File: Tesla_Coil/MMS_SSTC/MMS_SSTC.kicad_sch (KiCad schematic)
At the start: 57 parts, among them J1 Screw_Terminal_01x02, J2 Screw_Terminal_01x02, J3 Screw_Terminal_01x02, J4 Screw_Terminal_01x02, Q1 IRFP460APBF, U1 LM7812_TO220, U2 LM7805_TO220, U3 CD74HC14E, U4 UCC27524P, U5 NE555P

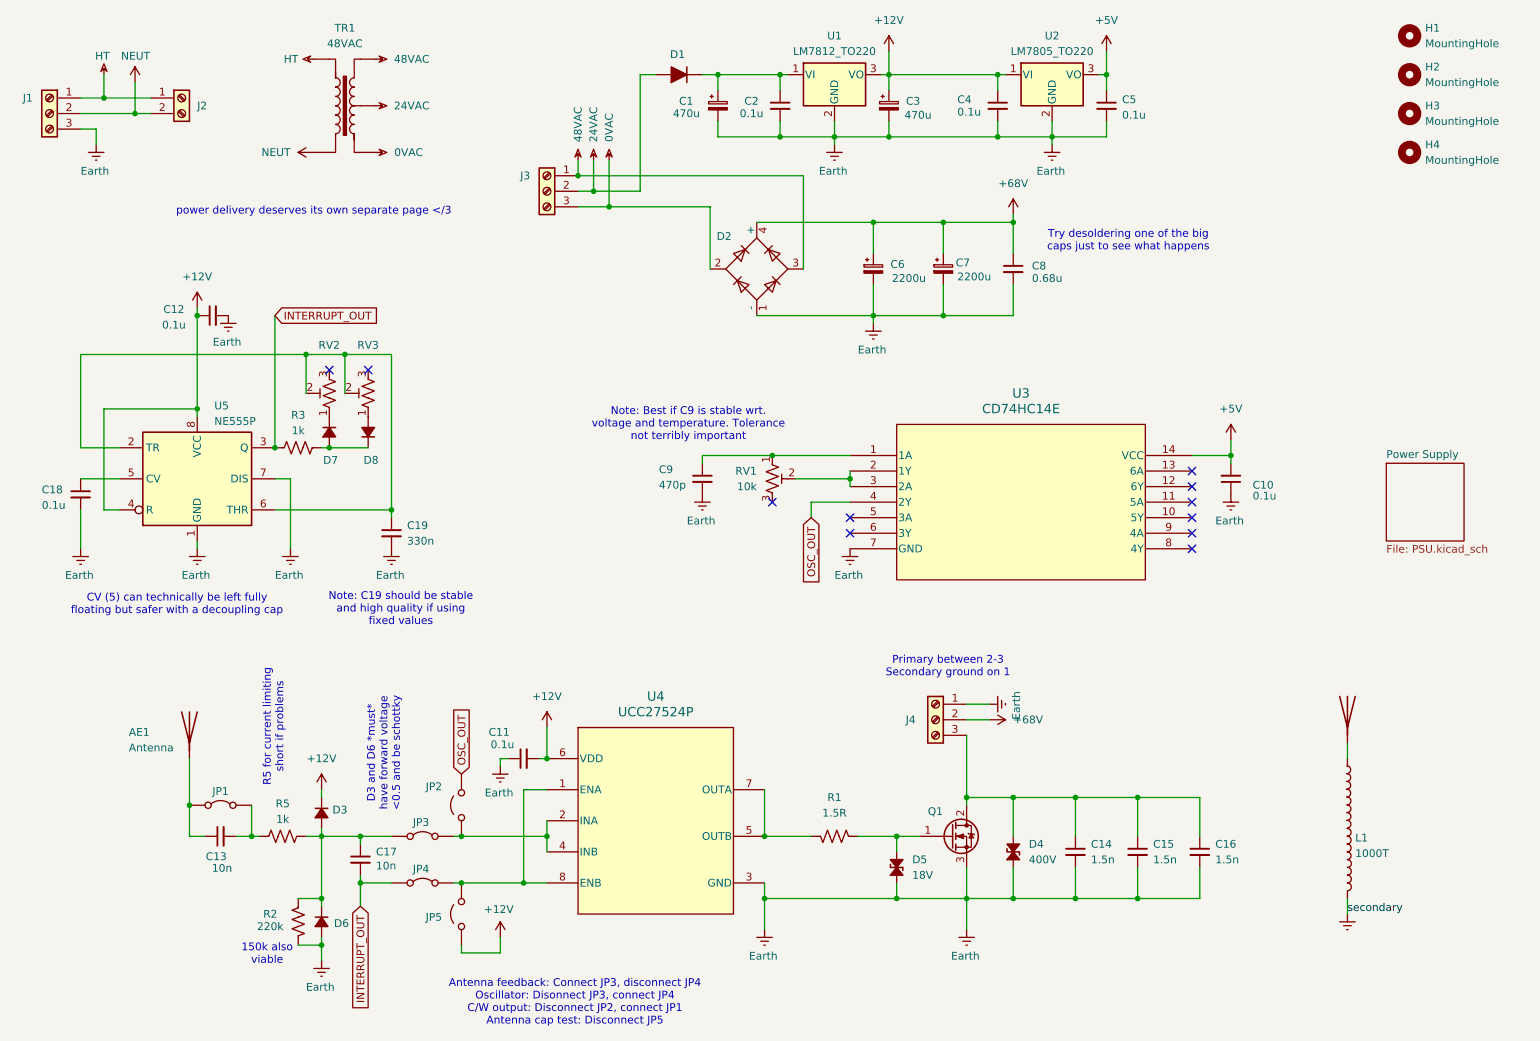
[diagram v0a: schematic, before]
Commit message: Begin work on final tesla coil design
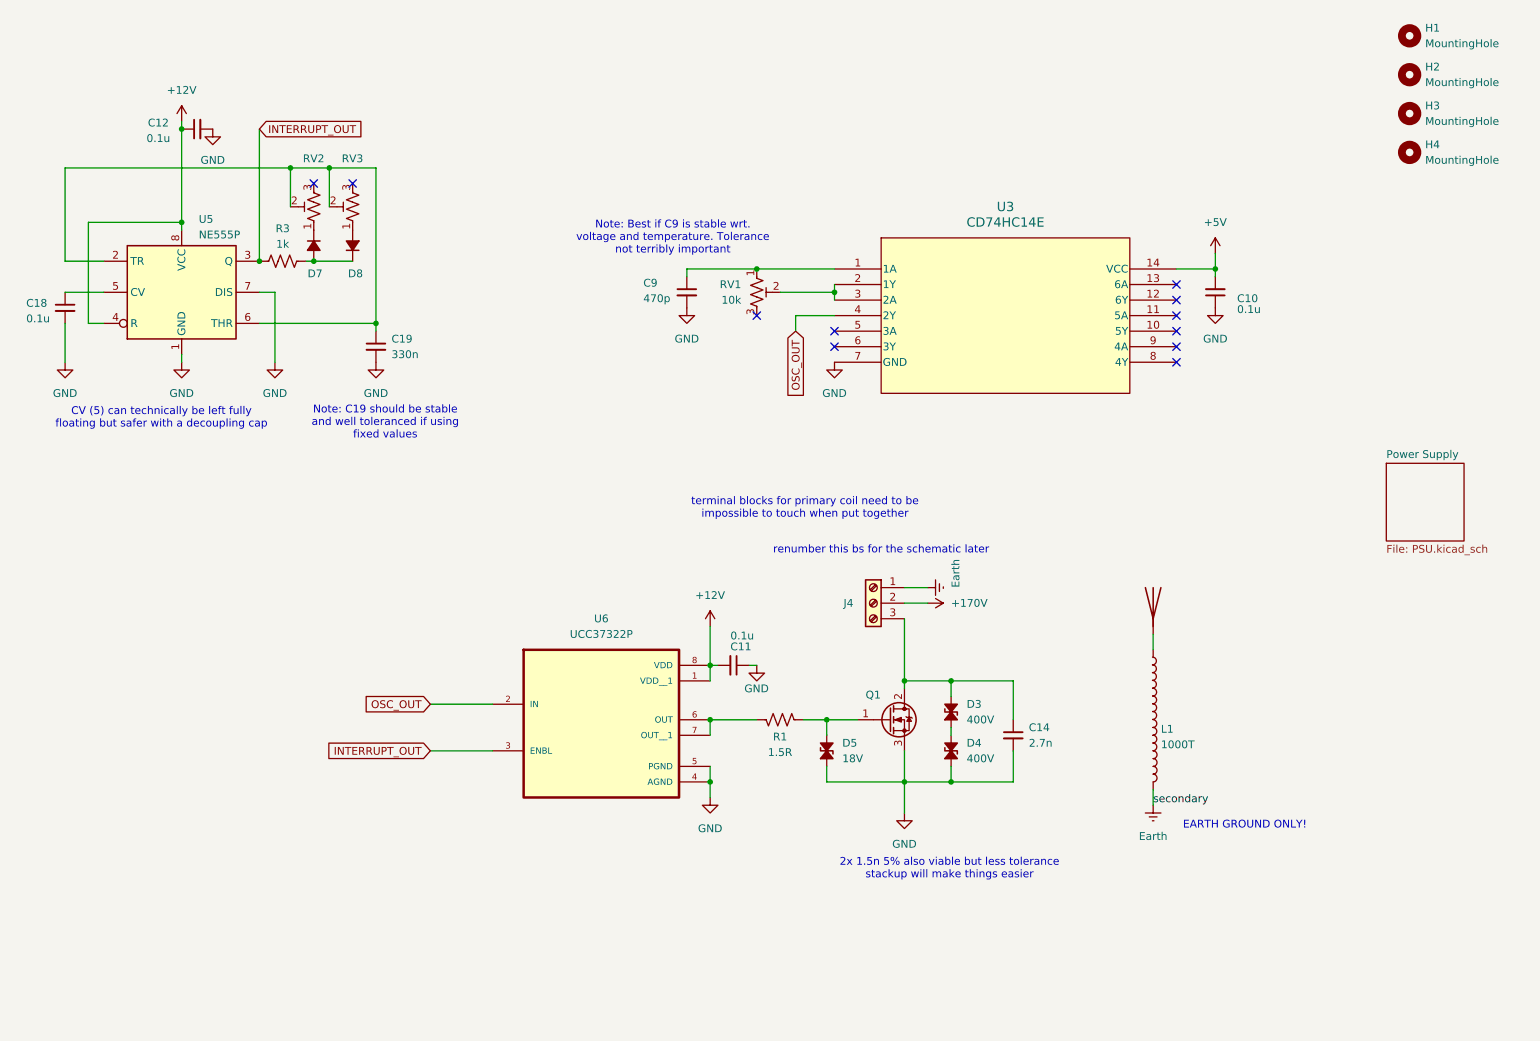
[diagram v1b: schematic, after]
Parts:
- removed AE1: Antenna, TestPoint:TestPoint_Keystone_5000-5004_Miniature, symbol Device:Antenna
- removed C1, C3: 470u, Capacitor_THT:CP_Radial_D12.5mm_P5.00mm, symbol Device:C_Polarized_Small
- removed C13, C17: 10n, Capacitor_THT:C_Disc_D5.0mm_W2.5mm_P2.50mm, symbol Device:C_Small
- removed C15, C16: 1.5n, Capacitor_THT:C_Rect_L13.0mm_W4.0mm_P10.00mm_FKS3_FKP3_MKS4, symbol Device:C_Small
- removed C2, C4, C5: 0.1u, Capacitor_THT:C_Disc_D3.0mm_W2.0mm_P2.50mm, symbol Device:C_Small
- removed C6, C7: 2200u, Capacitor_THT:CP_Radial_D25.0mm_P10.00mm_SnapIn, symbol Device:C_Polarized_Small
- removed C8: 0.68u, Capacitor_THT:C_Rect_L7.2mm_W5.5mm_P5.00mm_FKS2_FKP2_MKS2_MKP2, symbol Device:C_Small
- removed D1: D_Filled, Diode_THT:D_DO-41_SOD81_P7.62mm_Horizontal, symbol Device:D_Filled
- removed D2: B125C2300-1500A, Diode_THT:Diode_Bridge_Vishay_GBU, symbol Diode_Bridge:B125C2300-1500A
- removed D3, D6: ~, Diode_THT:D_DO-41_SOD81_P7.62mm_Horizontal, symbol Device:D_Small_Filled
- removed J1, J3: Screw_Terminal_01x02, locals:691137710003, symbol Connector:Screw_Terminal_01x03
- removed J2: Screw_Terminal_01x02, locals:691137710002, symbol Connector:Screw_Terminal_01x02
- removed JP1, JP3, JP4: Jumper_2_Bridged, TestPoint:TestPoint_Bridge_Pitch2.54mm_Drill0.7mm, symbol Jumper:Jumper_2_Bridged
- removed JP2, JP5: Jumper_2_Open, TestPoint:TestPoint_Bridge_Pitch2.54mm_Drill0.7mm, symbol Jumper:Jumper_2_Open
- removed R2: 220k, Resistor_THT:R_Axial_DIN0204_L3.6mm_D1.6mm_P5.08mm_Horizontal, symbol Device:R_US
- removed R5: 1k, Resistor_THT:R_Axial_DIN0204_L3.6mm_D1.6mm_P5.08mm_Horizontal, symbol Device:R_US
- removed TR1: 48VAC, symbol Transformer:TRANSF4
- removed U1: LM7812_TO220, Package_TO_SOT_THT:TO-220-3_Vertical, symbol Regulator_Linear:LM7812_TO220
- removed U2: LM7805_TO220, Package_TO_SOT_THT:TO-220-3_Vertical, symbol Regulator_Linear:LM7805_TO220
- removed U4: UCC27524P, Package_DIP:DIP-8_W7.62mm, symbol locals:UCC27524P
- added D3: 400V, Diode_THT:D_DO-27_P12.70mm_Horizontal, symbol Device:D_TVS_Small_Filled
- added U6: UCC37322P, UCC37322P:DIP794W45P254L959H508Q8, symbol locals:UCC37322P
- C14: value 1.5n -> 2.7n; DKPN 495-3205-ND -> 495-3223-ND
- Q1: value IRFP460APBF -> FQA8N100C; DKPN IRFP460APBF-ND -> FQA8N100CFS-ND
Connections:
- net +12V: now also U6.1 (VDD__1), U6.8 (VDD)
- net Earth: no longer C10.1, C11.1, C12.2, C14.2, C18.2, C19.2, C9.2, D4.1 (A1), D5.1 (A1), Q1.3 (S), U3.7 (GND), U5.1 (GND), U5.7 (DIS)
- net INTERRUPT_OUT: now also U6.3 (ENBL)
- net OSC_OUT: now also U6.2 (IN)
- net at R1.2: now also U6.6 (OUT), U6.7 (OUT__1)
- net at C14.1, J4.3 (Pin_3), Q1.2 (D): now also D3.2 (A2); no longer D4.2 (A2)
- net +68V renamed +170V
- new net: D3.1 (A1), D4.2 (A2)
- new net GND: C10.1, C11.1, C12.2, C14.2, C18.2, C19.2, C9.2, D4.1 (A1), D5.1 (A1), Q1.3 (S), U3.7 (GND), U5.1 (GND), U5.7 (DIS), U6.4 (AGND), U6.5 (PGND)
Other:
- note added: "2x 1.5n 5% also viable but less tolerance stackup will make things easier"
- note added: "EARTH GROUND ONLY!"
- note added: "Note: C19 should be stable and well toleranced if using fixed values"
- note added: "renumber this bs for the schematic later"
- note added: "terminal blocks for primary coil need to be impossible to touch when put together"
- note removed: "150k also viable"
- note removed: "Antenna feedback: Connect JP3, disconnect JP4 Oscillator: Disonnect JP3, connect JP4 C/W output: Disconnect JP2, connect JP1 Antenna cap test: Disconnect JP5"
- note removed: "D3 and D6 *must* have forward voltage <0.5 and be schottky"
- note removed: "Note: C19 should be stable and high quality if using fixed values"
- note removed: "Primary between 2-3 Secondary ground on 1"
- note removed: "R5 for current limiting short if problems"
- note removed: "Try desoldering one of the big caps just to see what happens"
- note removed: "power delivery deserves its own separate page </3"
- moved on the sheet: C10, C11, C12, C14, C18, C19, C9, D4, D5, D7, D8, J4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
